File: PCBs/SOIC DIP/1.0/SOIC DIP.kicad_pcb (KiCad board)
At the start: 2 copper layers, 13 x 14.5 mm, 4 parts, among them U1 OPA2134, U2 OPA2134

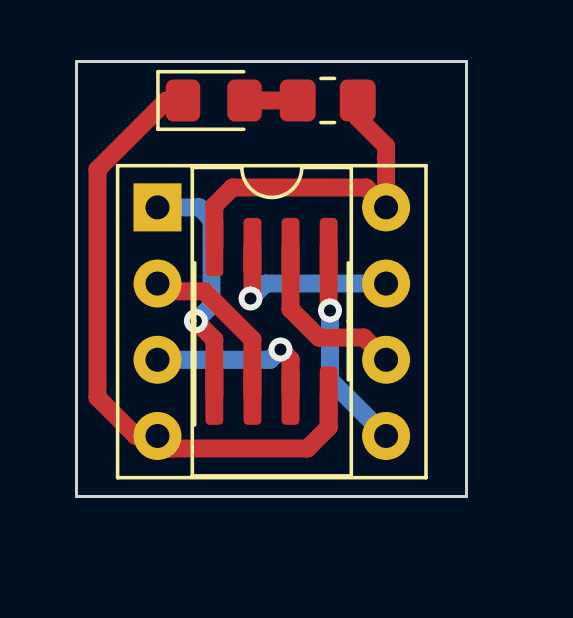
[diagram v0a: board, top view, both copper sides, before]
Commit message: Major updates
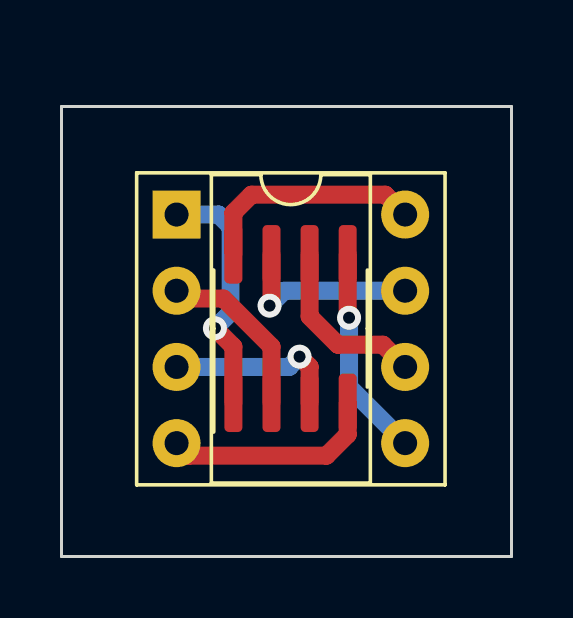
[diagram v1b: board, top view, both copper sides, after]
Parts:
- removed D1: LED, LED_SMD:LED_0805_2012Metric_Pad1.15x1.40mm_HandSolder
- removed R1: 6.5K, Resistor_SMD:R_0805_2012Metric_Pad1.20x1.40mm_HandSolder
- moved U1 0.68 mm to (138.8, 101.1)
- moved U2 0.68 mm to (142.6, 104.9)
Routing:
- net 4: track 21.2 -> 7.23 mm
- net 8: track 11.6 -> 7.63 mm
- net Net-(D1-Pad2): track 1.78 -> 0.00 mm
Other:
- board size 13 x 14.5 mm -> 15 x 15 mm
